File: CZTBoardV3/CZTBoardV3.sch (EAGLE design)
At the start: 37 parts, among them IC1 LD117AS33TR, IC2 LD117AS33TR, X6 GX16

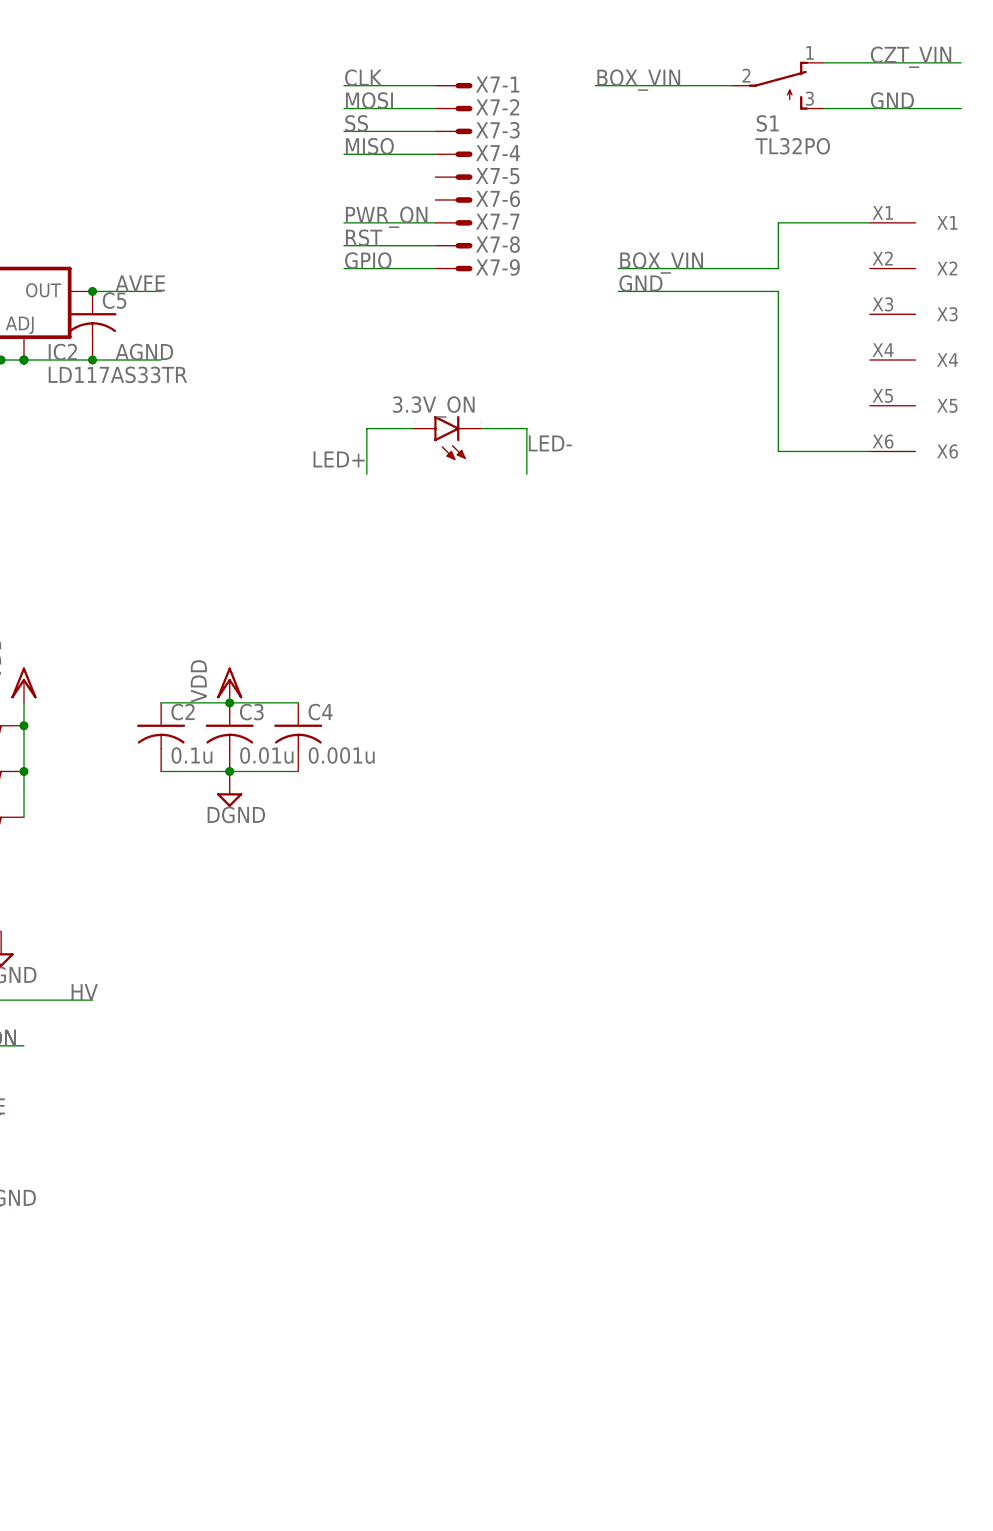
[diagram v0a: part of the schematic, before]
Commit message: Updated to final design and created output paths
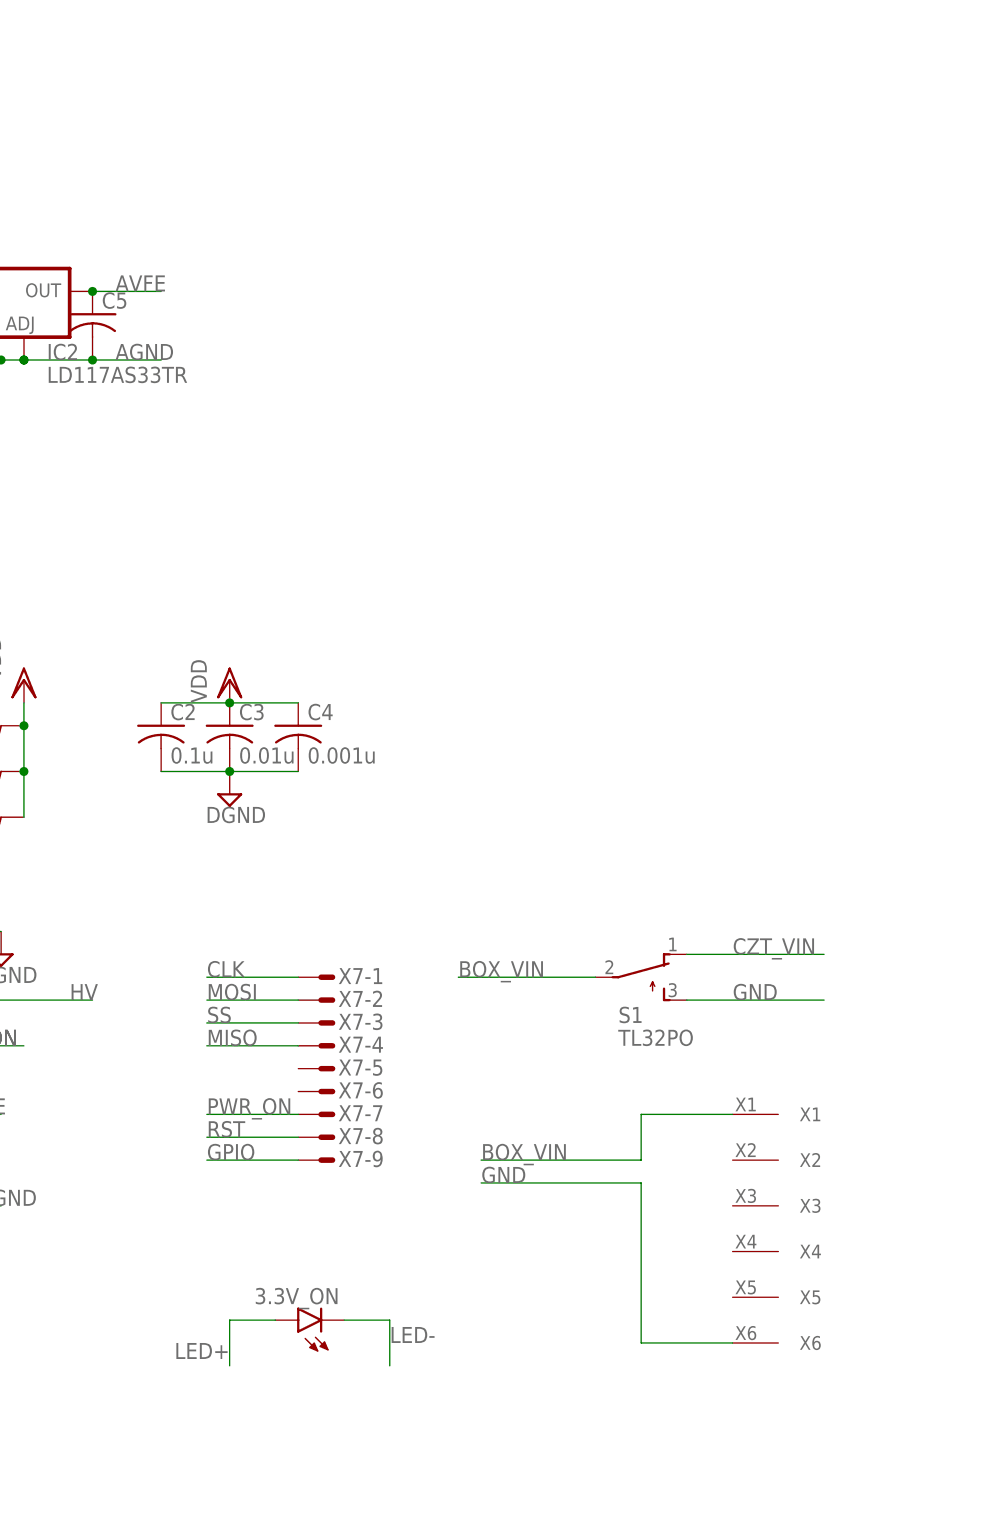
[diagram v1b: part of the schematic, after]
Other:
- moved on the sheet: 3.3V_ON, S1, X7-1, X7-2, X7-3, X7-4, X7-5, X7-6, X7-7, X7-8, X7-9
